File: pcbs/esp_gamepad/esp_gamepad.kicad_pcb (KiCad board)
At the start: 2 copper layers, 183 x 91.9 mm, 65 parts, among them J1 2.54mm, P1 USB_C_Plug_USB2.0, Q2 SI2300, SW1 SW_Push, SW10 SW_Push, SW11 SW_Push, SW12 SW_Push, SW13 SW_Push, SW14 DIP, SW2 SW_Push, SW3 SW_Push, SW4 SW_Push, SW5 SW_Push, SW6 SW_Push, SW7 SW_Push, SW8 SW_Push, SW9 SW_Push, U1 COM-09032, U2 IP5306, U5 LC709203FQH-02TWG, U7 COM-09032

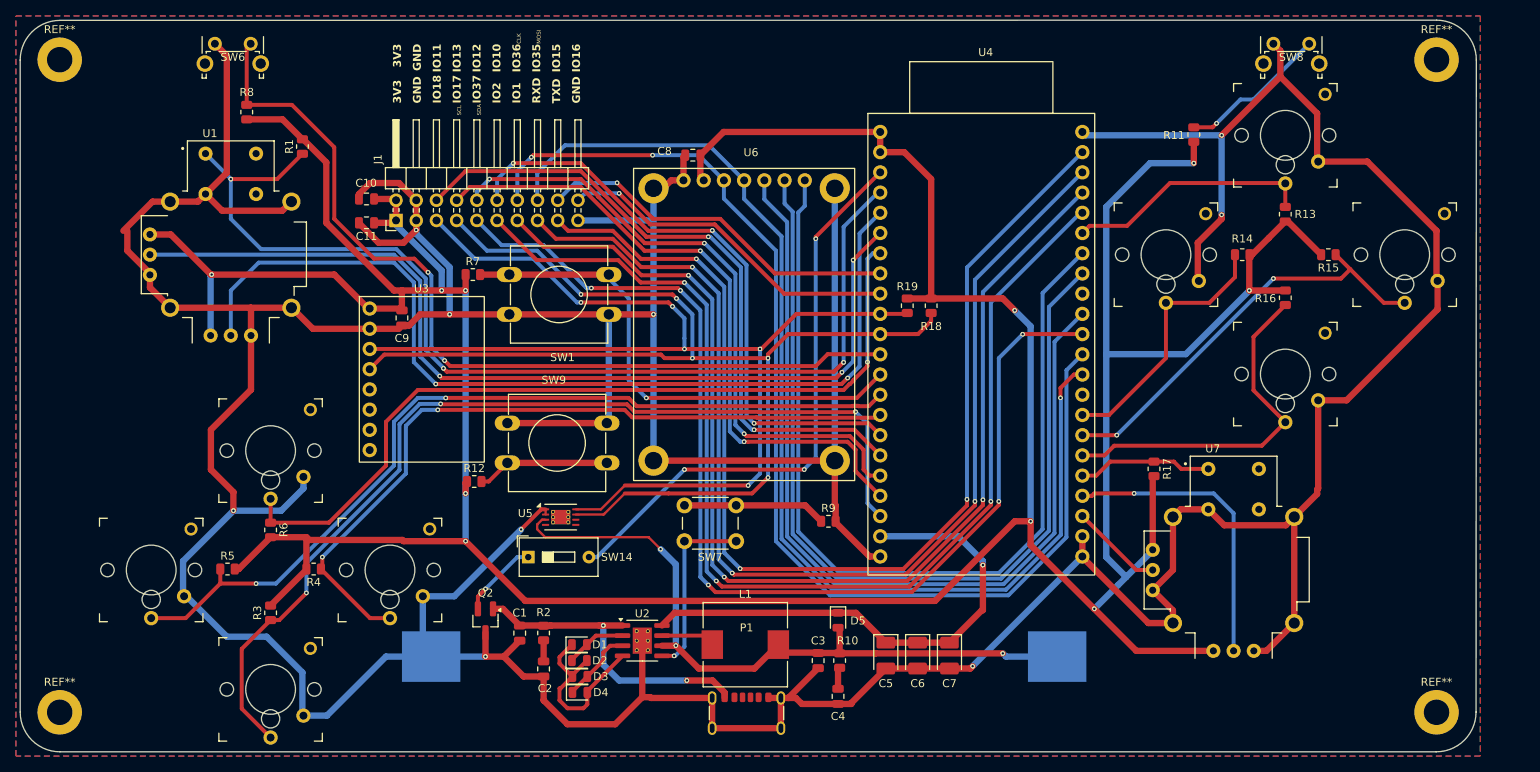
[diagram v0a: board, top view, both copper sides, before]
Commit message: pcb modification
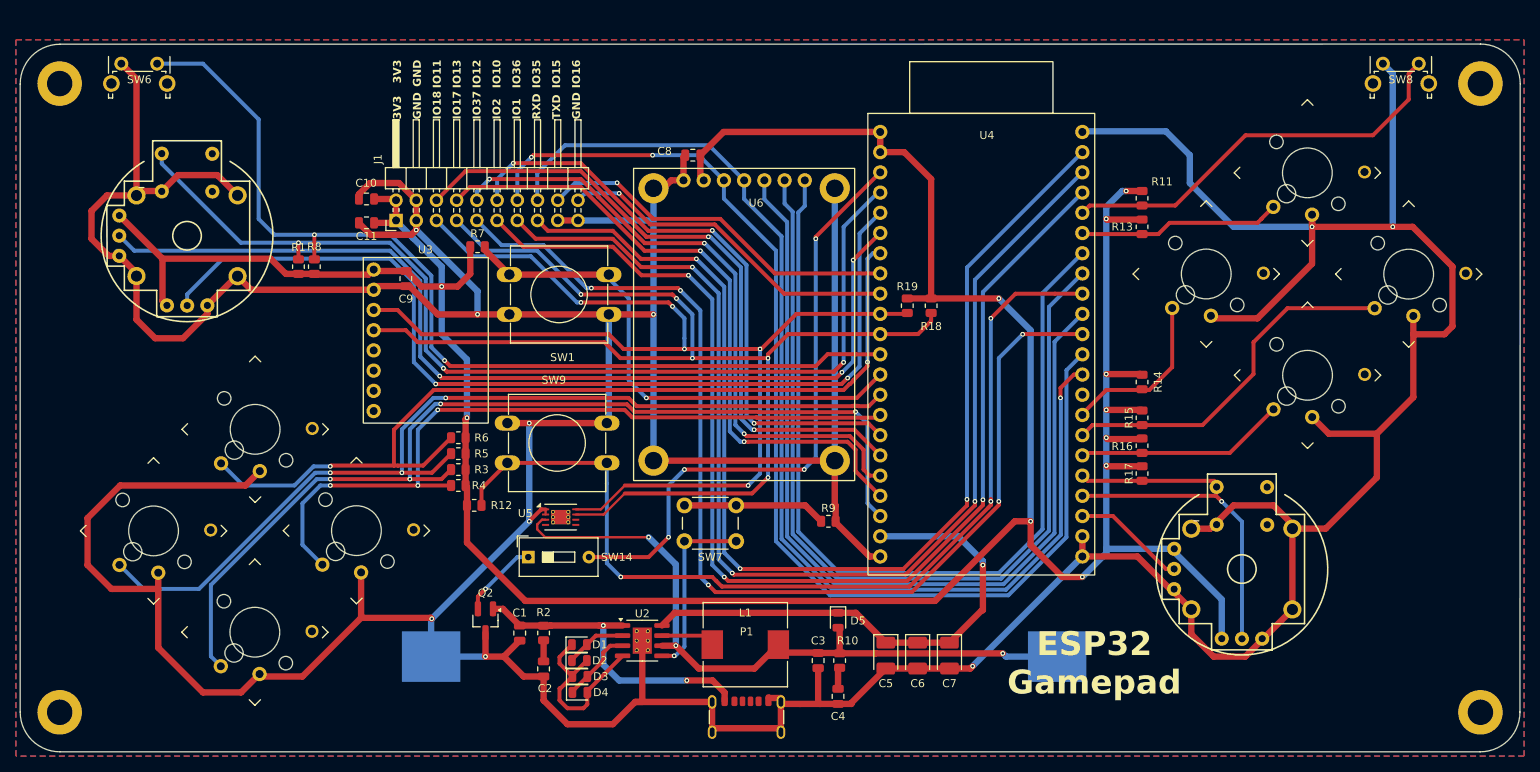
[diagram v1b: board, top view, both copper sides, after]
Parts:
- U1, U7: footprint Joystick:Joystick -> Joystick:PS4_joystick
- moved R5 32.4 mm to (115.6, 93.5)
- moved R15 31.1 mm to (201.5, 89.0), turned to 90 degrees
- moved R3 29.7 mm to (115.6, 95.5), turned to 0 degrees
- moved R6 26.3 mm to (115.6, 91.5), turned to 0 degrees
- moved R16 25.9 mm to (201.5, 92.5)
- moved R8 21.2 mm to (97.5, 70.0)
- moved R4 21.0 mm to (115.6, 97.5), turned to 0 degrees
- moved R14 20.4 mm to (201.5, 84.5), turned to 90 degrees
- moved R13 18.1 mm to (201.5, 65.0), turned to 90 degrees
- moved R1 15.1 mm to (95.5, 70.0), turned to -90 degrees
- moved SW8 14.0 mm to (231.8, 44.5)
- moved SW6 12.0 mm to (73.2, 44.5)
- moved R11 10.3 mm to (201.5, 61.4), turned to -90 degrees
- moved SW5 7.45 mm to (90.0, 115.9), turned to -45 degrees
- moved SW4 6.50 mm to (102.8, 103.2), turned to -45 degrees
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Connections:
- J1 pad 6: /IO2 -> /IO1
- J1 pad 7: /IO1 -> /RXD
- J1 pad 8: /RXD -> /TXD
- J1 pad 9: /TXD -> GND
- R11 pad 2: Net-(R11-Pad2) -> /IO2
- R12 pad 2: Net-(R12-Pad2) -> /IO39
- SW8 pad 2: Net-(R11-Pad2) -> /IO2
- SW9 pad 2: Net-(R12-Pad2) -> /IO39
- U4 pad 36: unconnected-(U4-IO39-Pad36) -> /IO39
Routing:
- net /IO39: track 0.00 -> 122.3 mm, vias 0 -> 3
- net /3V3: track 512.2 -> 392.1 mm, vias 10 -> 11
- net /IO2: track 146.6 -> 52.2 mm, vias 3 -> 0
- net GND: track 754.4 -> 796.7 mm, vias 9 -> 10
- net /IO47: track 45.3 -> 26.4 mm
- net Net-(R11-Pad2): track 18.8 -> 0.00 mm, vias 1 -> 0
- net Net-(R12-Pad2): track 16.7 -> 0.00 mm
- net /IO45: track 33.2 -> 21.3 mm
- net /IO8: track 112.2 -> 122.9 mm
- net /IO7: track 104.8 -> 115.3 mm, vias 1 -> 2
- net /IO46: track 109.2 -> 118.2 mm, vias 2 -> 3
- net /IO48: track 53.5 -> 45.7 mm, vias 2 -> 0
- net /IO42: track 31.1 -> 25.8 mm
- net /IO4: track 134.0 -> 129.1 mm
- net /IO6: track 118.7 -> 123.6 mm
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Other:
- board size 183 x 91.9 mm -> 188.5 x 88.9 mm
- board text added: "ESP32 Gamepad"
- board text added: "Made by: Nhien Nguyen"
- board text removed: "CLK"
- board text removed: "MOSI"
- board text removed: "SCL"
- board text removed: "SDA"
